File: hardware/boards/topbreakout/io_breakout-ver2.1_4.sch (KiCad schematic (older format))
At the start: 1 part, among them J4 ST7735_1.4

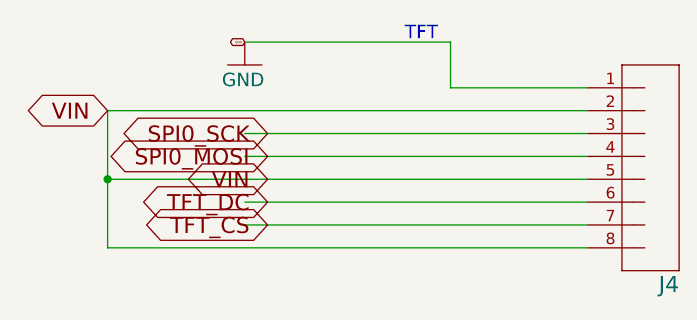
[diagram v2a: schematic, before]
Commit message: routed, ERC checks success
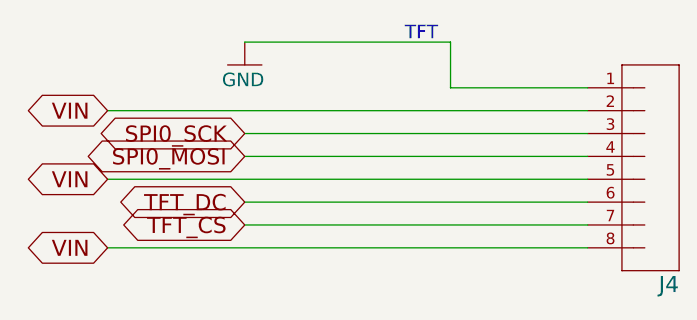
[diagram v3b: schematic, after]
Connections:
- wire segments 12 -> 10
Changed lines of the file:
@@
 Wire Wire Line
 	6200 3800 6800 3800
-Text GLabel 5300 3600 0    10   BiDi ~ 0
-GND
 Wire Wire Line
 	5300 4400 6800 4400
-Text GLabel 5400 4400 0    70   BiDi ~ 0
+Text GLabel 5300 4400 0    70   BiDi ~ 0
 TFT_CS
 Wire Wire Line
 	5300 4300 6800 4300
-Text GLabel 5400 4300 0    70   BiDi ~ 0
+Text GLabel 5300 4300 0    70   BiDi ~ 0
 TFT_DC
 Wire Wire Line
 	5300 4000 6800 4000
-Text GLabel 5400 4000 0    70   BiDi ~ 0
+Text GLabel 5300 4000 0    70   BiDi ~ 0
 SPI0_SCK
 Wire Wire Line
 	5300 4100 6800 4100
-Text GLabel 5400 4100 0    70   BiDi ~ 0
+Text GLabel 5300 4100 0    70   BiDi ~ 0
 SPI0_MOSI
-Wire Wire Line
-	6800 4200 4700 4200
 Wire Wire Line
 	6800 3900 4700 3900
 Wire Wire Line
-	4700 3900 4700 4200
-Wire Wire Line
-	4700 4200 4700 4500
-Wire Wire Line
 	6800 4500 4700 4500
-Text GLabel 5400 4200 0    70   BiDi ~ 0
-VIN
-Connection ~ 4700 4200
 Text GLabel 4700 3900 0    70   BiDi ~ 0
 VIN
@@
 Text Notes 6000 3600 0    59   ~ 0
 TFT
+Wire Wire Line
+	6800 4200 4700 4200
+Text GLabel 4700 4200 0    70   BiDi ~ 0
+VIN
+Text GLabel 4700 4500 0    70   BiDi ~ 0
+VIN
 $EndSCHEMATC
